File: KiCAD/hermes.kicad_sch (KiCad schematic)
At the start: 6 parts, among them U1 MPU-6500, U2 XIAO-RP2040-DIP

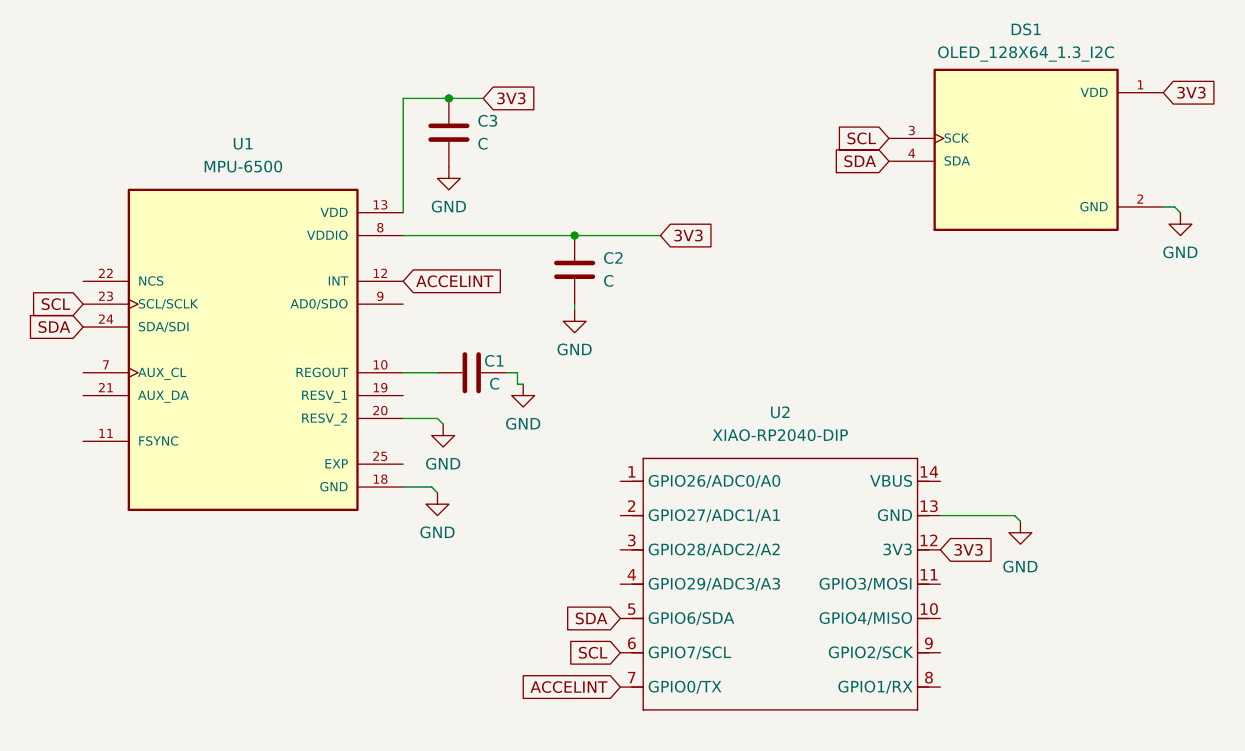
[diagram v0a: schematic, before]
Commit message: step 3 + 4
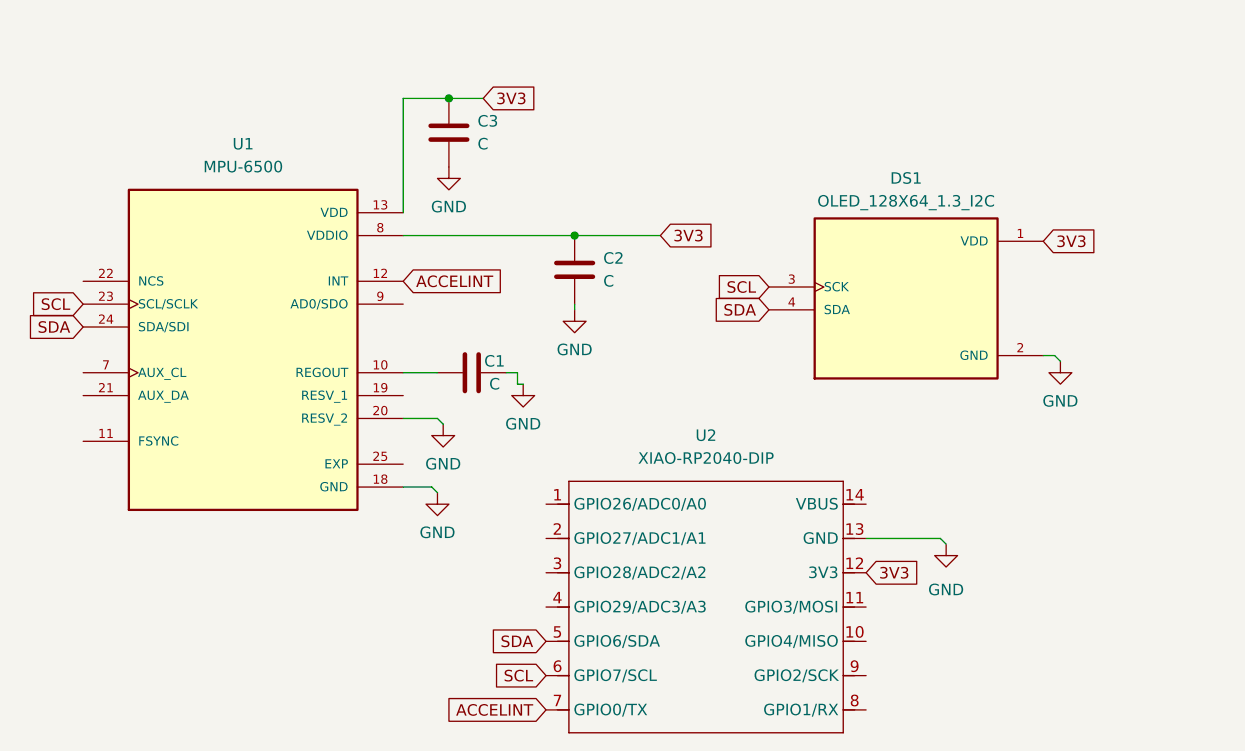
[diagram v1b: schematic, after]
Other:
- moved on the sheet: DS1, U2
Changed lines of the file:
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@@
 	(wire
 		(pts
-			(xy 148.59 107.315) (xy 149.225 107.95)
+			(xy 140.335 109.855) (xy 140.97 110.49)
 		)
 		(stroke
@@
 	(wire
 		(pts
-			(xy 140.335 107.315) (xy 148.59 107.315)
+			(xy 132.08 109.855) (xy 140.335 109.855)
 		)
 		(stroke
@@
 	(wire
 		(pts
-			(xy 165.1 73.025) (xy 166.37 73.025)
+			(xy 151.765 89.535) (xy 153.035 89.535)
 		)
 		(stroke
@@
 	(wire
 		(pts
-			(xy 166.37 73.025) (xy 167.005 73.66)
+			(xy 153.035 89.535) (xy 153.67 90.17)
 		)
 		(stroke
@@
 	(global_label "SCL"
 		(shape input)
-		(at 104.775 122.555 180)
+		(at 96.52 125.095 180)
 		(fields_autoplaced yes)
 		(effects
@@
 		)
 		(property "Intersheetrefs" "${INTERSHEET_REFS}"
-			(at 98.2822 122.555 0)
+			(at 90.0272 125.095 0)
 			(effects
 				(font
@@
 	(global_label "3V3"
 		(shape input)
-		(at 165.1 60.325 0)
+		(at 151.765 76.835 0)
 		(fields_autoplaced yes)
 		(effects
@@
 		)
 		(property "Intersheetrefs" "${INTERSHEET_REFS}"
-			(at 171.5928 60.325 0)
+			(at 158.2578 76.835 0)
 			(effects
 				(font
@@
 	(global_label "SDA"
 		(shape input)
-		(at 134.62 67.945 180)
+		(at 121.285 84.455 180)
 		(fields_autoplaced yes)
 		(effects
@@
 		)
 		(property "Intersheetrefs" "${INTERSHEET_REFS}"
-			(at 128.0667 67.945 0)
+			(at 114.7317 84.455 0)
 			(effects
 				(font
@@
 	(global_label "ACCELINT"
 		(shape input)
-		(at 104.775 126.365 180)
+		(at 96.52 128.905 180)
 		(fields_autoplaced yes)
 		(effects
@@
 		)
 		(property "Intersheetrefs" "${INTERSHEET_REFS}"
-			(at 93.0812 126.365 0)
+			(at 84.8262 128.905 0)
 			(effects
 				(font
@@
 	(global_label "SDA"
 		(shape input)
-		(at 104.775 118.745 180)
+		(at 96.52 121.285 180)
 		(fields_autoplaced yes)
 		(effects
@@
 		)
 		(property "Intersheetrefs" "${INTERSHEET_REFS}"
-			(at 98.2217 118.745 0)
+			(at 89.9667 121.285 0)
 			(effects
 				(font
@@
 	(global_label "3V3"
 		(shape input)
-		(at 140.335 111.125 0)
+		(at 132.08 113.665 0)
 		(fields_autoplaced yes)
 		(effects
@@
 		)
 		(property "Intersheetrefs" "${INTERSHEET_REFS}"
-			(at 146.8278 111.125 0)
+			(at 138.5728 113.665 0)
 			(effects
 				(font
@@
 	(global_label "SCL"
 		(shape input)
-		(at 134.62 65.405 180)
+		(at 121.285 81.915 180)
 		(fields_autoplaced yes)
 		(effects
@@
 		)
 		(property "Intersheetrefs" "${INTERSHEET_REFS}"
-			(at 128.1272 65.405 0)
+			(at 114.7922 81.915 0)
 			(effects
 				(font
@@
 	(symbol
 		(lib_id "power:GND")
-		(at 149.225 107.95 0)
+		(at 140.97 110.49 0)
 		(unit 1)
 		(exclude_from_sim no)
@@
 		(fields_autoplaced yes)
 		(property "Reference" "#PWR03"
-			(at 149.225 114.3 0)
+			(at 140.97 116.84 0)
 			(effects
 				(font
@@
 		)
 		(property "Value" "GND"
-			(at 149.225 113.03 0)
+			(at 140.97 115.57 0)
 			(effects
 				(font
@@
 		)
 		(property "Footprint" ""
-			(at 149.225 107.95 0)
+			(at 140.97 110.49 0)
 			(effects
 				(font
@@
 		)
 		(property "Datasheet" ""
-			(at 149.225 107.95 0)
+			(at 140.97 110.49 0)
 			(effects
 				(font
@@
 		)
 		(property "Description" "Power symbol creates a global label with name \"GND\" , ground"
-			(at 149.225 107.95 0)
+			(at 140.97 110.49 0)
 			(effects
 				(font
@@
 		(on_board yes)
 		(dnp no)
-		(fields_autoplaced yes)
 		(property "Reference" "#PWR04"
 			(at 93.98 99.06 0)
@@
 	(symbol
 		(lib_id "Seeed_Studio_XIAO_Series:XIAO-RP2040-DIP")
-		(at 108.585 98.425 0)
+		(at 100.33 100.965 0)
 		(unit 1)
 		(exclude_from_sim no)
@@
 		(on_board yes)
 		(dnp no)
-		(fields_autoplaced yes)
 		(property "Reference" "U2"
-			(at 122.555 95.885 0)
+			(at 114.3 98.425 0)
 			(effects
 				(font
@@
 		)
 		(property "Value" "XIAO-RP2040-DIP"
-			(at 122.555 98.425 0)
+			(at 114.3 100.965 0)
 			(effects
 				(font
@@
 		)
 		(property "Footprint" "footprints:XIAO-RP2040-DIP"
-			(at 123.063 130.683 0)
+			(at 114.808 133.223 0)
 			(effects
 				(font
@@
 		)
 		(property "Datasheet" ""
-			(at 108.585 98.425 0)
+			(at 100.33 100.965 0)
 			(effects
 				(font
@@
 		)
 		(property "Description" ""
-			(at 108.585 98.425 0)
+			(at 100.33 100.965 0)
 			(effects
 				(font
@@
 	(symbol
 		(lib_id "power:GND")
-		(at 167.005 73.66 0)
+		(at 153.67 90.17 0)
 		(unit 1)
 		(exclude_from_sim no)
@@
 		(fields_autoplaced yes)
 		(property "Reference" "#PWR07"
-			(at 167.005 80.01 0)
+			(at 153.67 96.52 0)
 			(effects
 				(font
@@
 		)
 		(property "Value" "GND"
-			(at 167.005 78.105 0)
+			(at 153.67 94.615 0)
 			(effects
 				(font
@@
 		)
 		(property "Footprint" ""
-			(at 167.005 73.66 0)
+			(at 153.67 90.17 0)
 			(effects
 				(font
@@
 		)
 		(property "Datasheet" ""
-			(at 167.005 73.66 0)
+			(at 153.67 90.17 0)
 			(effects
 				(font
@@
 		)
 		(property "Description" "Power symbol creates a global label with name \"GND\" , ground"
-			(at 167.005 73.66 0)
+			(at 153.67 90.17 0)
 			(effects
 				(font
@@
 	(symbol
 		(lib_id "OLED_128X64_1.3_I2C:OLED_128X64_1.3_I2C")
-		(at 149.86 67.945 0)
+		(at 136.525 84.455 0)
 		(unit 1)
 		(exclude_from_sim no)
@@
 		(fields_autoplaced yes)
 		(property "Reference" "DS1"
-			(at 149.86 53.34 0)
+			(at 136.525 69.85 0)
 			(effects
 				(font
@@
 		)
 		(property "Value" "OLED_128X64_1.3_I2C"
-			(at 149.86 55.88 0)
+			(at 136.525 72.39 0)
 			(effects
 				(font
@@
 		)
 		(property "Footprint" "footprints:128x64OLED"
-			(at 149.86 67.945 0)
+			(at 136.525 84.455 0)
 			(effects
 				(font
@@
 		)
 		(property "Datasheet" ""
-			(at 149.86 67.945 0)
+			(at 136.525 84.455 0)
 			(effects
 				(font
@@
 		)
 		(property "Description" ""
-			(at 149.86 67.945 0)
+			(at 136.525 84.455 0)
 			(effects
 				(font
@@
 		)
 		(property "MF" "UNIVERSAL-SOLDER Electronics Ltd"
-			(at 149.86 67.945 0)
+			(at 136.525 84.455 0)
 			(effects
 				(font
@@
 		)
 		(property "Description_1" "Non-Touch Graphic LCD Display Module Transmissive White OLED, Monochrome I2C 1.3 (33.02mm) 128 x 64"
-			(at 149.86 67.945 0)
+			(at 136.525 84.455 0)
 			(effects
 				(font
@@
 		)
 		(property "Package" "None"
-			(at 149.86 67.945 0)
+			(at 136.525 84.455 0)
 			(effects
 				(font
@@
 		)
 		(property "Price" "None"
-			(at 149.86 67.945 0)
+			(at 136.525 84.455 0)
 			(effects
 				(font
@@
 		)
 		(property "Check_prices" "https://www.snapeda.com/parts/OLED%20128x64%201.3%22%20I2C/UNIVERSAL-SOLDER+Electronics+Ltd/view-part/?ref=eda"
-			(at 149.86 67.945 0)
+			(at 136.525 84.455 0)
 			(effects
 				(font
@@
 		)
 		(property "STANDARD" "Manufacturer Recommendations"
-			(at 149.86 67.945 0)
+			(at 136.525 84.455 0)
 			(effects
 				(font
@@
 		)
 		(property "PARTREV" "NA"
-			(at 149.86 67.945 0)
+			(at 136.525 84.455 0)
 			(effects
 				(font
@@
 		)
 		(property "SnapEDA_Link" "https://www.snapeda.com/parts/OLED%20128x64%201.3%22%20I2C/UNIVERSAL-SOLDER+Electronics+Ltd/view-part/?ref=snap"
-			(at 149.86 67.945 0)
+			(at 136.525 84.455 0)
 			(effects
 				(font
@@
 		)
 		(property "MP" "OLED 128x64 1.3&quot; I2C"
-			(at 149.86 67.945 0)
+			(at 136.525 84.455 0)
 			(effects
 				(font
@@
 		)
 		(property "Availability" "Not in stock"
-			(at 149.86 67.945 0)
+			(at 136.525 84.455 0)
 			(effects
 				(font
@@
 		)
 		(property "MANUFACTURER" "UNIVERSAL-SOLDER Electronics Ltd"
-			(at 149.86 67.945 0)
-			(effects
-				(font
+			(at 136.525 84.455 0)
+			(effects
+				(font
